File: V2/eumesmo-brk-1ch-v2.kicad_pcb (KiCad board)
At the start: 2 copper layers, 22 x 28 mm, 3 parts, among them J1 RJ45, J2 1x4P 5,08 SCREW

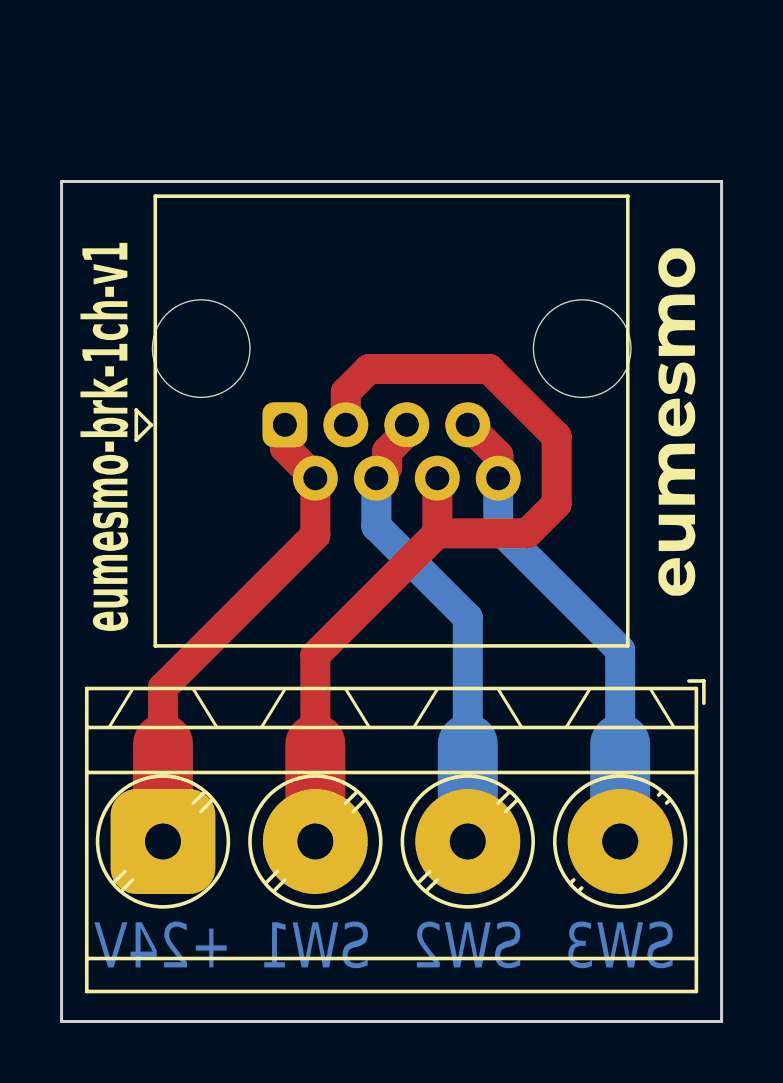
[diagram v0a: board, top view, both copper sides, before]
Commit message: V2.0.0 created
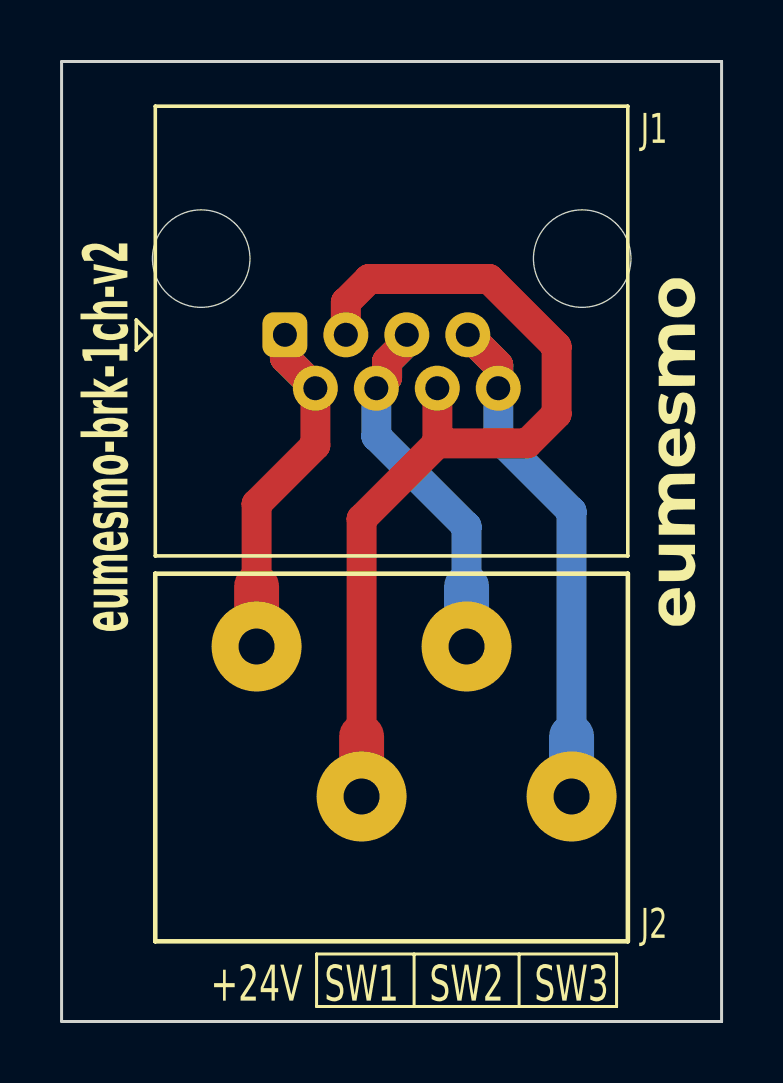
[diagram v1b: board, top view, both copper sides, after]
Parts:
- J2: value 1x4P 5,08 SCREW -> 250-204; footprint Tales:TerminalBlock_Dibo_DB128L-5.08-4P_1x04_P5.08mm_Horizontal -> Tales:TerminalBlock_Wago_250-204_1x04_P3.5mm_45Degree
- moved J2 4.07 mm to (141.8, 110.0)
- moved J1 3.00 mm to (141.0, 98.0)
- moved G*** 1.00 mm to (148.5, 101.0)
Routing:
- net /+24V: track 18.6 -> 13.8 mm
- net /SW2: track 17.8 -> 14.3 mm
- net /SW1: track 29.8 -> 30.6 mm
- net /SW3: track 18.2 -> 19.0 mm
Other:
- board size 22 x 28 mm -> 22 x 32 mm
- board text added: "eumesmo-brk-1ch-v2"
- board text removed: "eumesmo-brk-1ch-v1"
